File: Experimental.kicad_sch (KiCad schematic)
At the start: 12 parts, among them J1 MX128-5.0-04P-GN01-Cu-Y-A, J3 MX128-5.0-04P-GN01-Cu-Y-A, J4 MX128-5.0-04P-GN01-Cu-Y-A, J7 MX128-5.0-04P-GN01-Cu-Y-A, J9 MX128-5.0-04P-GN01-Cu-Y-A

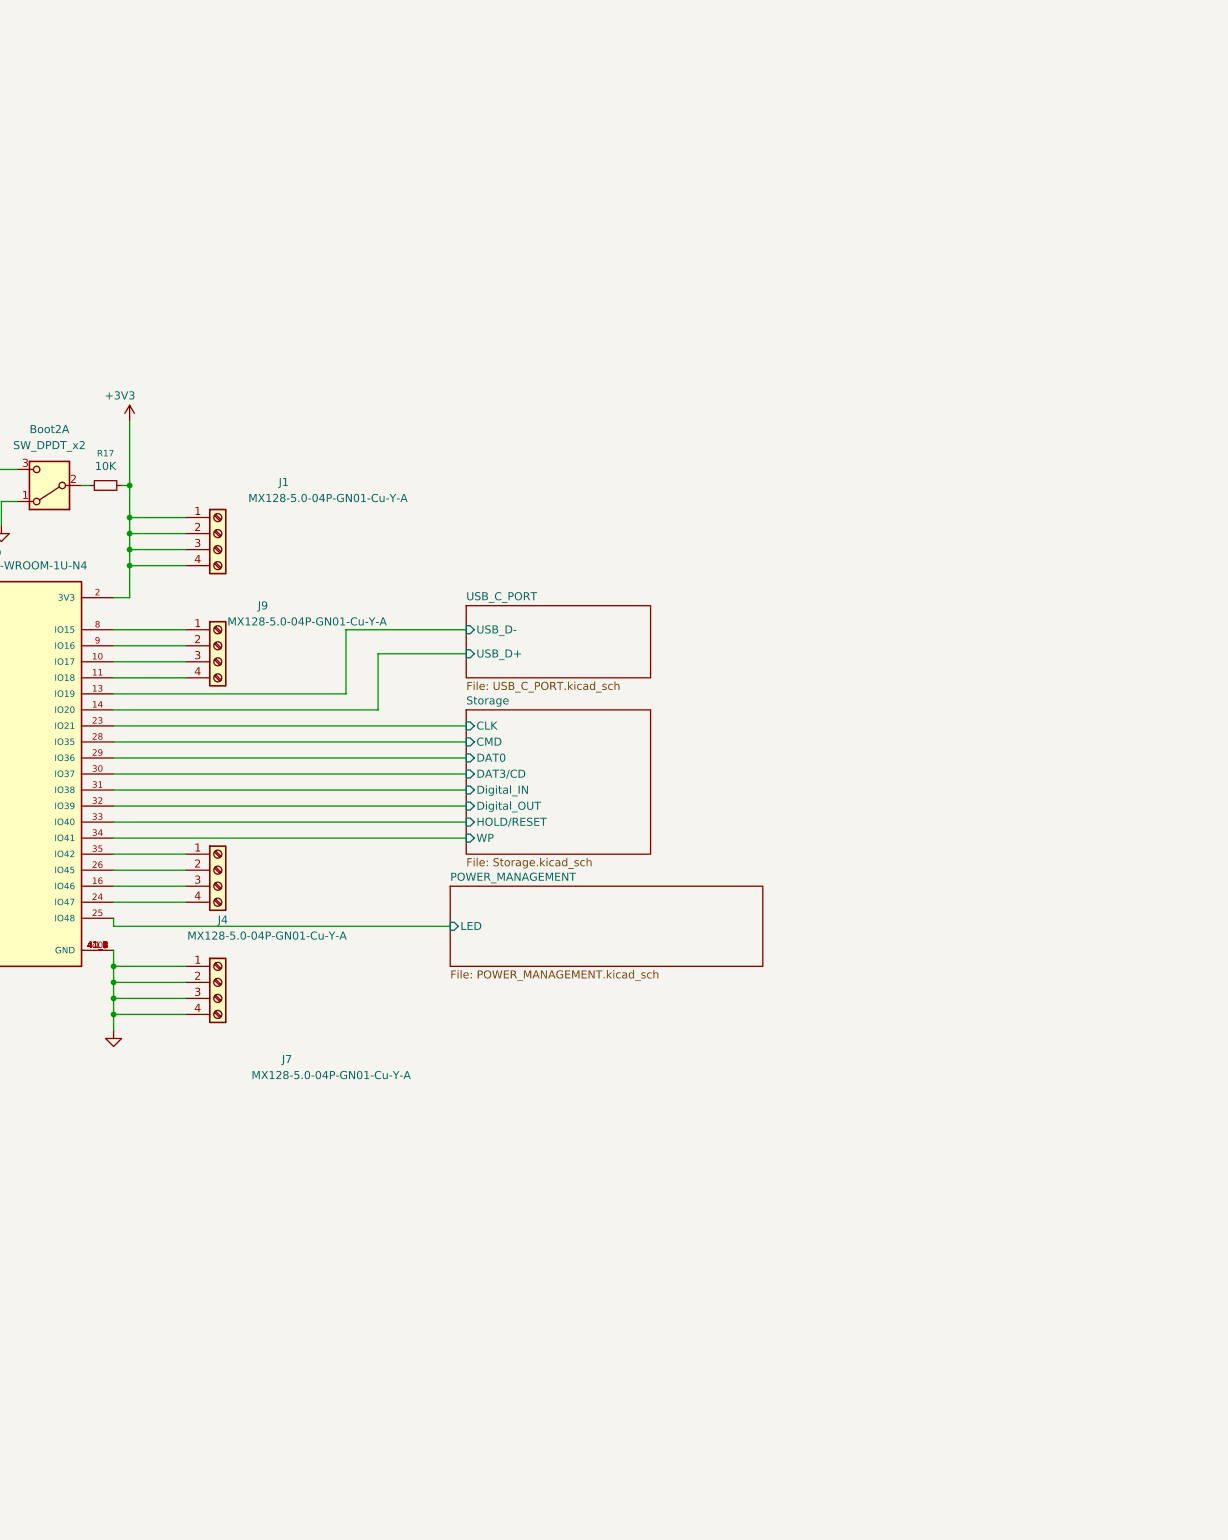
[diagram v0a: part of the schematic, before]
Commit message: Tweaks and readability
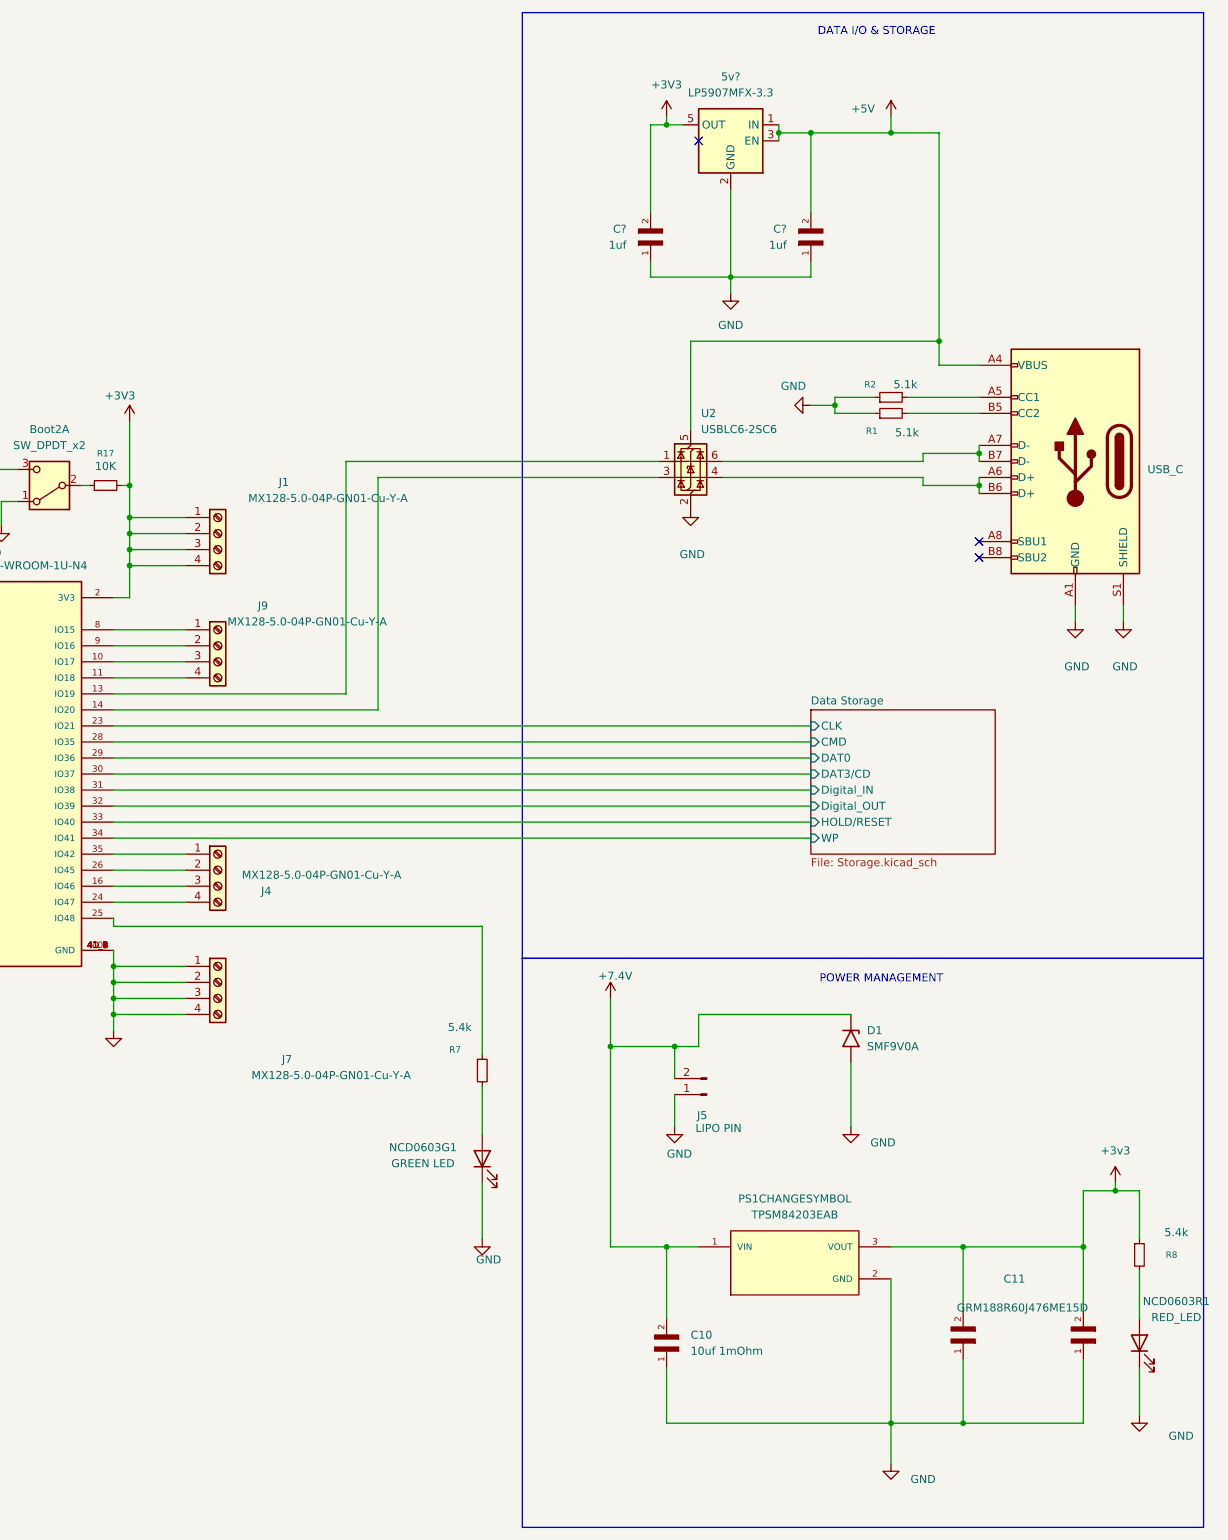
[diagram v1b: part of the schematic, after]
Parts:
- added 5v?: LP5907MFX-3.3, Package_TO_SOT_SMD:SOT-23-5, symbol Regulator_Linear:LP5907MFX-3.3
- added C10: 10uf 1mOhm, Capacitor_SMD:C_0805_2012Metric, symbol MCASE168SB7105MTNA01:MCASE168SB7105MTNA01
- added C11: GRM188R60J476ME15D, Capacitor:EEEHP1H4R7P, symbol MCASE168SB7105MTNA01:MCASE168SB7105MTNA01
- added C12: GRM188R60J476ME15D, Capacitor:CAPC1608X100N, symbol MCASE168SB7105MTNA01:MCASE168SB7105MTNA01
- added C? (x2): 1uf, Capacitor_SMD:C_0402_1005Metric, symbol MCASE168SB7105MTNA01:MCASE168SB7105MTNA01
- added D1: SMF9V0A, Diode_SMD:D_SMF, symbol Diode:SMF9V0A
- added J5: LIPO PIN, Connector_JST:JST_PH_B2B-PH-K_1x02_P2.00mm_Vertical, symbol Connector:Conn_01x02_Pin
- added NCD0603G1: GREEN LED, LED_SMD:LED_0603_1608Metric, symbol Device:LED
- added NCD0603R1: RED_LED, LED_SMD:LED_0603_1608Metric, symbol Device:LED
- added PS1CHANGESYMBOL: TPSM84203EAB, footprints:CONV_TPSM84205EAB, symbol TPSM84205EAB:TPSM84205EAB
- added PowerUpload1: USB_C, Connector_USB:USB_C_Receptacle_GCT_USB4105-xx-A_16P_TopMnt_Horizontal, symbol Connector:USB_C_Receptacle_USB2.0_16P
- added R1, R2: 5.1k, Resistor:R0402, symbol Device:R_Small
- added R7, R8: 5.4k, Resistor_SMD:R_0402_1005Metric, symbol Device:R_Small
- added U2: USBLC6-2SC6, Package_TO_SOT_SMD:SOT-23-6, symbol Power_Protection:USBLC6-2SC6
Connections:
- net +3V3: now also 5v?.5 (OUT), C?.2
- net GND: now also 5v?.2 (GND), C10.1, C11.1, C12.1, C?.1, C?.1, D1.2 (A2), J5.1 (7.4v), NCD0603G1.1 (K), NCD0603R1.1 (K), PS1CHANGESYMBOL.2 (GND), PowerUpload1.A1 (GND), PowerUpload1.A12 (GND), PowerUpload1.B1 (GND), PowerUpload1.B12 (GND), PowerUpload1.S1 (SHIELD), R1.1, R2.1, U2.2 (GND)
- net POWER_MANAGEMENT/LED: no longer names the net of ESP32S3.25 (IO48)
- net POWER_MANAGEMENT/LED: now also R7.1
- net USB_C_PORT/USB_D+: no longer names the net of ESP32S3.14 (IO20)
- net USB_C_PORT/USB_D+: now also U2.3 (I/O2)
- net USB_C_PORT/USB_D-: no longer names the net of ESP32S3.13 (IO19)
- net USB_C_PORT/USB_D-: now also U2.1 (I/O1)
- new net: PowerUpload1.B5 (CC2), R1.2
- new net: NCD0603G1.2 (A), R7.2
- new net: PowerUpload1.A5 (CC1), R2.2
- new net: PowerUpload1.A6 (D+), PowerUpload1.B6 (D+), U2.4 (I/O2)
- new net: PowerUpload1.A7 (D-), PowerUpload1.B7 (D-), U2.6 (I/O1)
- new net: NCD0603R1.2 (A), R8.2
- new net +3v3: C11.2, C12.2, PS1CHANGESYMBOL.3 (VOUT), R8.1
- new net +5V: 5v?.1 (IN), 5v?.3 (EN), C?.2, PowerUpload1.A4 (VBUS), PowerUpload1.A9 (VBUS), PowerUpload1.B4 (VBUS), PowerUpload1.B9 (VBUS), U2.5 (VBUS)
- new net +7.4V: C10.2, D1.1 (A1), J5.2 (GND), PS1CHANGESYMBOL.1 (VIN)
- no-connect marks 0 -> 3
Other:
- sheet Storage renamed Data Storage
- removed sheet POWER_MANAGEMENT
- removed sheet USB_C_PORT
- note added: "DATA I/O & STORAGE"
- note added: "POWER MANAGEMENT"

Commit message: Undo hiearchical layer
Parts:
- added Barometer1: BMP388, BMP388:PQFN50P200X200X80-10N, symbol BMP388:BMP388
- added C1: 6800 UF, Capacitor:CAPPRD500W85D1250H3700, symbol EEU-FR1A682B:EEU-FR1A682B
- added C3, C4, C5, C7, C8, C9: 100nF, Capacitor:CAPC1608X90N, symbol MCASE168SB7105MTNA01:MCASE168SB7105MTNA01
- added C6: 1uF, Capacitor_SMD:C_0402_1005Metric, symbol MCASE168SB7105MTNA01:MCASE168SB7105MTNA01
- added D?: RED LED, LED_SMD:LED_0402_1005Metric, symbol Device:LED
- added IMU6axis1: LSM6DSOXTR, LSM6DSOX:PQFN50P250X300X86-14N, symbol LSM6DSOX:LSM6DSOX
- added J7CHECK: 20279-001E-03, footprints:IPEX_20279-001E-03, symbol 20279-001E-03:20279-001E-03
- added J? (x2): Screw_Terminal, TerminalBlock:TerminalBlock_MaiXu_MX126-5.0-02P_1x02_P5.00mm, symbol Connector:Screw_Terminal_01x02
- added Magnometer1: LIS3MDLTR, Package_LGA:LGA-12_2x2mm_P0.5mm, symbol Sensor_Magnetic:LIS3MDL
- added Q2_32mW?, Q? (x2): AO3400A, Package_TO_SOT_SMD:SOT-23, symbol Transistor_FET:AO3400A
- added R10, R11, R12, R13, R21, R9, R? (x3): 10k, Resistor:R0402, symbol Device:R_Small
- added R? (x2): 2200, Resistor:R0402, symbol Device:R_Small
- added R? (x2): 330, Resistor:R0402, symbol Device:R_Small
- added R?: 1 ohm, 20W, Resistor:R0402, symbol Device:R_Small
- added R?: 147, Resistor:R0402, symbol Device:R_Small
- added SDCard1: Micro_SD_Card, Connector_Card:microSD_HC_Hirose_DM3AT-SF-PEJM5, symbol Connector:Micro_SD_Card_Det_Hirose_DM3AT
- added U1: NEO-M8N, RF_GPS:ublox_NEO, symbol RF_GPS:NEO-M8N
- added WSON-8-Flash1: U10, Package_SON:WSON-8-1EP_8x6mm_P1.27mm_EP3.4x4.3mm, symbol Memory_Flash:W25Q128JVE
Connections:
- net PYRO_N_MOSFET_A1/Continuity Checker is gone; now on net GND: ESP32S3.19 (IO11)
- net +3V3: now also Barometer1.1 (VDDIO), Barometer1.10 (VDD), Barometer1.6 (CSB), C4.2, C5.2, C6.1, C7.1, C8.1, C9.1, IMU6axis1.5 (VDDIO), IMU6axis1.8 (VDD), Magnometer1.5 (Vdd), Magnometer1.6 (Vdd_IO), R10.2, R11.2, R12.2, R9.2, SDCard1.4 (VDD), U1.2 (D_SEL), U1.23 (VCC), WSON-8-Flash1.8 (VCC)
- net +7.4V: now also Q?.3 (D)
- net GND: now also ESP32S3.17 (IO9), Barometer1.3 (VSS), Barometer1.8 (VSS), Barometer1.9 (VSS), C1.2 (-), C3.2, C4.1, C5.1, C6.2, C7.2, C8.2, C9.2, D?.1 (K), IMU6axis1.2 (SDX), IMU6axis1.3 (SCX), IMU6axis1.6 (GND), IMU6axis1.7 (GND), J7CHECK.2, J7CHECK.3, Magnometer1.12 (GND), Magnometer1.2 (GND), Magnometer1.3 (GND), Q2_32mW?.3 (D), Q?.3 (D), R13.2, R21.1, R?.1, R?.1, R?.1, R?.1, SDCard1.11 (SHIELD), SDCard1.6 (VSS), U1.10 (GND), U1.12 (GND), U1.13 (GND), U1.24 (GND), WSON-8-Flash1.4 (GND), WSON-8-Flash1.9 (EP)
- net Data Storage/CLK: no longer names the net of ESP32S3.23 (IO21)
- net Data Storage/CLK: now also SDCard1.2 (DAT3/CD)
- net Data Storage/CMD: no longer names the net of ESP32S3.28 (IO35)
- net Data Storage/CMD: now also SDCard1.3 (CMD)
- net Data Storage/DAT0: no longer names the net of ESP32S3.29 (IO36)
- net Data Storage/DAT0: now also SDCard1.7 (DAT0)
- net Data Storage/DAT3/CD: no longer names the net of ESP32S3.30 (IO37)
- net Data Storage/DAT3/CD: now also SDCard1.5 (CLK), WSON-8-Flash1.6 (CLK)
- net Data Storage/Digital_IN: no longer names the net of ESP32S3.31 (IO38)
- net Data Storage/Digital_IN: now also WSON-8-Flash1.5 (DI/IO_{0})
- net Data Storage/Digital_OUT: no longer names the net of ESP32S3.32 (IO39)
- net Data Storage/Digital_OUT: now also WSON-8-Flash1.2 (DO/IO_{1})
- net Data Storage/HOLD/RESET: no longer names the net of ESP32S3.33 (IO40)
- net Data Storage/HOLD/RESET: now also WSON-8-Flash1.3 (~{WP}/IO_{2})
- net Data Storage/WP: no longer names the net of ESP32S3.34 (IO41)
- net Data Storage/WP: now also WSON-8-Flash1.7 (~{HOLD}/~{RESET}/IO_{3})
- net NEO-M8N-GPS/GPS_RESET: no longer names the net of ESP32S3.39 (IO1)
- net NEO-M8N-GPS/GPS_RESET: now also U1.8 (~{RESET})
- net NEO-M8N-GPS/GPS_RX: no longer names the net of ESP32S3.37 (TXD0)
- net NEO-M8N-GPS/GPS_RX: now also U1.21 (RXD/SPI_MOSI)
- net NEO-M8N-GPS/GPS_TX: no longer names the net of ESP32S3.36 (RXD0)
- net NEO-M8N-GPS/GPS_TX: now also U1.20 (TXD/SPI_MISO)
- net NEO-M8N-GPS/LNA_EN: no longer names the net of ESP32S3.38 (IO2)
- net NEO-M8N-GPS/LNA_EN: now also U1.14 (LNA_EN)
- net NEO-M8N-GPS/TIMEPULSE: no longer names the net of ESP32S3.15 (IO3)
- net NEO-M8N-GPS/TIMEPULSE: now also U1.3 (TIMEPULSE)
- net PYRO_N_MOSFET_A1/Charge_Pyro: no longer names the net of ESP32S3.18 (IO10)
- net PYRO_N_MOSFET_A1/Charge_Pyro: now also R?.1
- net PYRO_N_MOSFET_A1/Continuity Checker2: no longer names the net of ESP32S3.21 (IO13)
- net PYRO_N_MOSFET_A1/Continuity Checker2: now also R6.1, Barometer1.4 (SDI), IMU6axis1.14 (SDA), Magnometer1.11 (SDA/SDI/SDO)
- net PYRO_N_MOSFET_A1/Pyro: no longer names the net of ESP32S3.20 (IO12)
- net PYRO_N_MOSFET_A1/Pyro: now also Q?.1 (G)
- net PYRO_N_MOSFET_A1/Pyro2: no longer names the net of ESP32S3.22 (IO14)
- net PYRO_N_MOSFET_A1/Pyro2: now also R3.1, Barometer1.2 (SCK), IMU6axis1.13 (SCL), Magnometer1.1 (SCL/SPC)
- removed net Sensors_I2C_BUS/SCL: ESP32S3.17 (IO9), R3.1
- net Sensors_I2C_BUS/SDA: no longer names the net of ESP32S3.12 (IO8)
- net Sensors_I2C_BUS/SDA: now also R?.1; no longer R6.1
- new net: Q?.1 (G), R?.2, R?.2
- new net: J?.2 (Pin_2), Q?.2 (S), R?.2
- new net: D?.2 (A), R?.1
- new net: Q?.2 (S), R?.2, R?.2
- new net: R13.1, WSON-8-Flash1.1 (~{CS})
- new net: Barometer1.5 (SDO), R21.2
- new net: IMU6axis1.12 (CS), R10.1
- new net: Magnometer1.10 (~{CS}), R11.1
- new net: Q2_32mW?.1 (G), R?.2, R?.2
- new net: Magnometer1.9 (SDO/SA1), R12.1
- new net: J?.1 (Pin_1), J?.1 (Pin_1), R?.1, R?.2
- new net: J7CHECK.1, U1.11 (RF_IN)
- new net: IMU6axis1.1 (SDO/SA0), R9.1
- new net: C3.1, Magnometer1.4 (C1)
- new net: J?.2 (Pin_2), Q2_32mW?.2 (S), R?.2
- new net: C1.1 (+), R?.1
- no-connect marks 3 -> 23
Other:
- removed sheet Data Storage
- removed sheet NEO-M8N-GPS
- removed sheet PYRO_N_MOSFET_A1
- removed sheet Sensors_I2C_BUS
- note added: "CHARGEPYRO"
- note added: "CONTINUITY1"
- note added: "CONTINUITY2"
- note added: "DATA STORAGE"
- note added: "GPS M8N"
- note added: "PYRO CIRCUIT, N-FET LOW-SWITCH"
- note added: "PYRO1"
- note added: "PYRO2"
- note added: "SENSORS, IMU, MAGNO, BARO"
- moved on the sheet: 5v?, C10, C11, C?, D1, J5, NCD0603G1, NCD0603R1, PS1CHANGESYMBOL, R1, R2, R3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
